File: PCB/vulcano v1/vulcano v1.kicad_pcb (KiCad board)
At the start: 2 copper layers, 4 parts, among them J1 Screw_Terminal_01x02, J2 Screw_Terminal_01x02, J3 conector t, U1 DOIT-ESP32-DEVKIT-V1

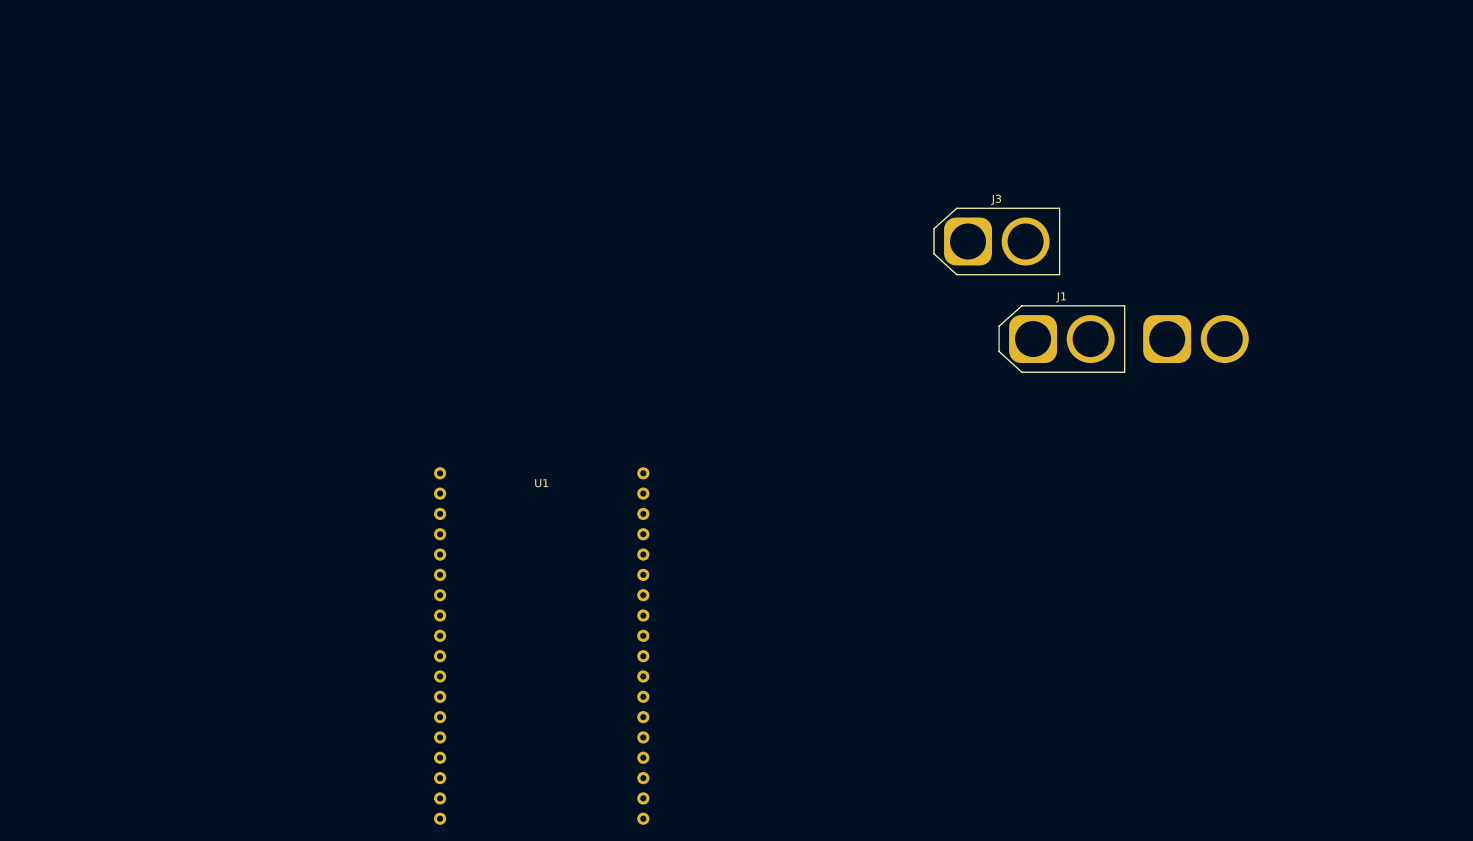
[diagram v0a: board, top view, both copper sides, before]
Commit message: placa principal
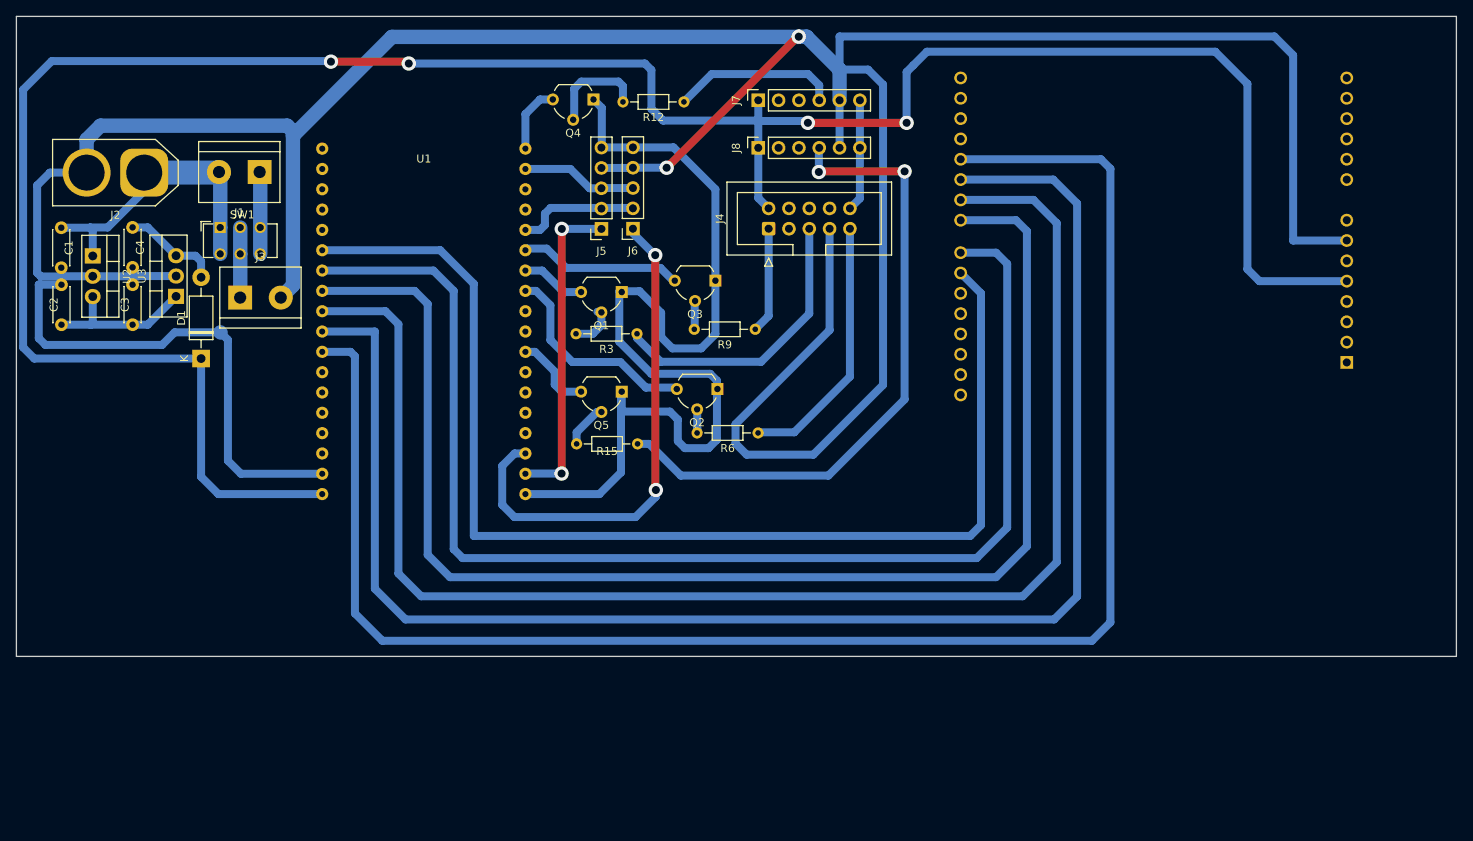
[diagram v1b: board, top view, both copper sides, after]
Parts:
- added A1: Arduino_UNO_R2, Module:Arduino_UNO_R2, B.Cu at (210.4, 77.6)
- added C1: 0.33uF, Capacitor_THT:C_Disc_D4.3mm_W1.9mm_P5.00mm, F.Cu at (49.7, 60.8)
- added C2: 0.1uF, Capacitor_THT:C_Disc_D4.3mm_W1.9mm_P5.00mm, F.Cu at (49.7, 72.9)
- added C3: 0.33uF, Capacitor_THT:C_Disc_D4.3mm_W1.9mm_P5.00mm, F.Cu at (58.6, 72.9)
- added C4: 0.1uF, Capacitor_THT:C_Disc_D4.3mm_W1.9mm_P5.00mm, F.Cu at (58.6, 60.7)
- added D1: 1N4007, Diode_THT:D_DO-41_SOD81_P10.16mm_Horizontal, F.Cu at (67.2, 77.1)
- added J4: Conn_02x05_Counter_Clockwise, Connector_IDC:IDC-Header_2x05_P2.54mm_Vertical, F.Cu at (138.1, 60.9)
- added J5: Conn_01x05_Pin, Connector_PinSocket_2.54mm:PinSocket_1x05_P2.54mm_Vertical, F.Cu at (117.2, 60.9)
- added J6: Conn_01x05_Pin, Connector_PinSocket_2.54mm:PinSocket_1x05_P2.54mm_Vertical, F.Cu at (121.1, 60.9)
- added J7: Conn_01x06_Pin, Connector_PinSocket_2.54mm:PinSocket_1x06_P2.54mm_Vertical, F.Cu at (136.8, 44.8)
- added J8: Conn_01x06_Pin, Connector_PinSocket_2.54mm:PinSocket_1x06_P2.54mm_Vertical, F.Cu at (136.8, 50.8)
- added Q1: BC547, Package_TO_SOT_THT:TO-92_Wide, F.Cu at (119.7, 68.8)
- added Q2: BC547, Package_TO_SOT_THT:TO-92_Wide, F.Cu at (131.7, 80.9)
- added Q3: BC547, Package_TO_SOT_THT:TO-92_Wide, F.Cu at (131.4, 67.4)
- added Q4: BC547, Package_TO_SOT_THT:TO-92_Wide, F.Cu at (116.2, 44.7)
- added Q5: BC547, Package_TO_SOT_THT:TO-92_Wide, F.Cu at (119.7, 81.3)
- added R12: 4k7, Resistor_THT:R_Axial_DIN0204_L3.6mm_D1.6mm_P7.62mm_Horizontal, F.Cu at (127.5, 45.0)
- added R15: 4k7, Resistor_THT:R_Axial_DIN0204_L3.6mm_D1.6mm_P7.62mm_Horizontal, F.Cu at (121.7, 87.8)
- added R3: 4k7, Resistor_THT:R_Axial_DIN0204_L3.6mm_D1.6mm_P7.62mm_Horizontal, F.Cu at (121.6, 74.0)
- added R6: 4k7, Resistor_THT:R_Axial_DIN0204_L3.6mm_D1.6mm_P7.62mm_Horizontal, F.Cu at (136.8, 86.4)
- added R9: 4k7, Resistor_THT:R_Axial_DIN0204_L3.6mm_D1.6mm_P7.62mm_Horizontal, F.Cu at (136.4, 73.5)
- added SW1: SW_SPDT, Button_Switch_THT:SW_CuK_JS202011CQN_DPDT_Straight, F.Cu at (69.5, 60.7)
- added U2: LM7809_TO220, Package_TO_SOT_THT:TO-220-3_Vertical, F.Cu at (53.6, 64.3)
- added U3: LM7806_TO220, Package_TO_SOT_THT:TO-220-3_Vertical, F.Cu at (64.0, 69.3)
- J1: footprint Connector_AMASS:AMASS_XT60-F_1x02_P7.20mm_Vertical -> TerminalBlock:TerminalBlock_bornier-2_P5.08mm
- J2: moved to F.Cu
- J3: value conector t -> Screw_Terminal_01x02; footprint Connector_AMASS:AMASS_XT60-F_1x02_P7.20mm_Vertical -> TerminalBlock:TerminalBlock_bornier-2_P5.08mm
- moved J2 129.6 mm to (60.0, 53.9), turned to 180 degrees
- moved J1 98.9 mm to (74.5, 53.8), turned to 180 degrees
- moved J3 91.3 mm to (72.0, 69.5)
- moved U1 43.2 mm to (95.0, 48.3)
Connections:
- net Net-(J1-Pin_2) renamed +12V
- J1 pad 1: GND -> Net-(J1-Pin_1)
- J2 pad 2: VCC -> GND
- U1 pad 10: unconnected-(U1-GPIO27_ADC2-CH7_RTC-GPIO17-Pad10) -> PWMA
- U1 pad 11: unconnected-(U1-GPIO14_ADC2-CH6_HSPI-CLK_RTC-GPIO16-Pad11) -> BIN1
- U1 pad 17: unconnected-(U1-GND-Pad17) -> GND
- U1 pad 18: unconnected-(U1-VIN-Pad18) -> +5V
- U1 pad 19: unconnected-(U1-3V3-Pad19) -> +3.3V
- U1 pad 20: unconnected-(U1-GPIO6_SCK/CLK-Pad20) -> X_SHUT_2
- U1 pad 21: unconnected-(U1-GPIO7_SDO/SD0-Pad21) -> X_SHUT_1
- U1 pad 26: unconnected-(U1-GPIO4_ADC2-CH0_RTC-GPIO10-Pad26) -> SENSOR_5_PIN
- U1 pad 29: unconnected-(U1-GPIO5_VSPI-CS0-Pad29) -> SENSOR_2_PIN
- U1 pad 30: unconnected-(U1-GPIO18_VSPI-CLK-Pad30) -> SENSOR_1_PIN
- U1 pad 31: unconnected-(U1-GPIO19_VSPI-MISO-Pad31) -> SENSOR_3_PIN
- U1 pad 32: unconnected-(U1-GPIO21_I2C-SDA-Pad32) -> SDA
- U1 pad 35: unconnected-(U1-GPIO22_I2C-SCL-Pad35) -> SCL
- U1 pad 36: unconnected-(U1-GPIO23_VSPI-MOSI-Pad36) -> SENSOR_4_PIN
- U1 pad 6: unconnected-(U1-GPIO32_ADC1-CH4_RTC-GPIO9-Pad6) -> BIN2
- U1 pad 7: unconnected-(U1-GPIO33_ADC1-CH5_RTC-GPIO8-Pad7) -> AIN2
- U1 pad 8: unconnected-(U1-GPIO25_ADC2-CH8_DAC1_RTC-GPIO6-Pad8) -> AIN1
- U1 pad 9: unconnected-(U1-GPIO26_ADC2-CH9_DAC2_RTC-GPIO7-Pad9) -> PWMB
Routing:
- net GND: track 0.00 -> 461.8 mm, vias 0 -> 2
- net +5V: track 0.00 -> 305.7 mm, vias 0 -> 4
- net BIN1: track 0.00 -> 209.2 mm
- net PWMA: track 0.00 -> 194.2 mm
- net PWMB: track 0.00 -> 182.2 mm
- net AIN1: track 0.00 -> 171.1 mm
- net AIN2: track 0.00 -> 160.4 mm
- net BIN2: track 0.00 -> 148.7 mm
- net +3.3V: track 0.00 -> 127.7 mm
- net RX_1: track 0.00 -> 81.3 mm, vias 0 -> 2
- net X_SHUT_1: track 0.00 -> 64.0 mm, vias 0 -> 2
- net X_SHUT_2: track 0.00 -> 40.1 mm, vias 0 -> 2
- net +12V: track 0.00 -> 37.9 mm
- net Sensores: track 0.00 -> 36.4 mm
- net Sensores_2: track 0.00 -> 32.9 mm
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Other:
- board outline added: 180 x 80 mm
